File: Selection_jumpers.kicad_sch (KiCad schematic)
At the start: 7 parts, among them J10 U2RS485_TX, J17 U2RS485_DE_~{RE}, J17 U2RS485_RX, J6 R4_TX, J7 R4_RX

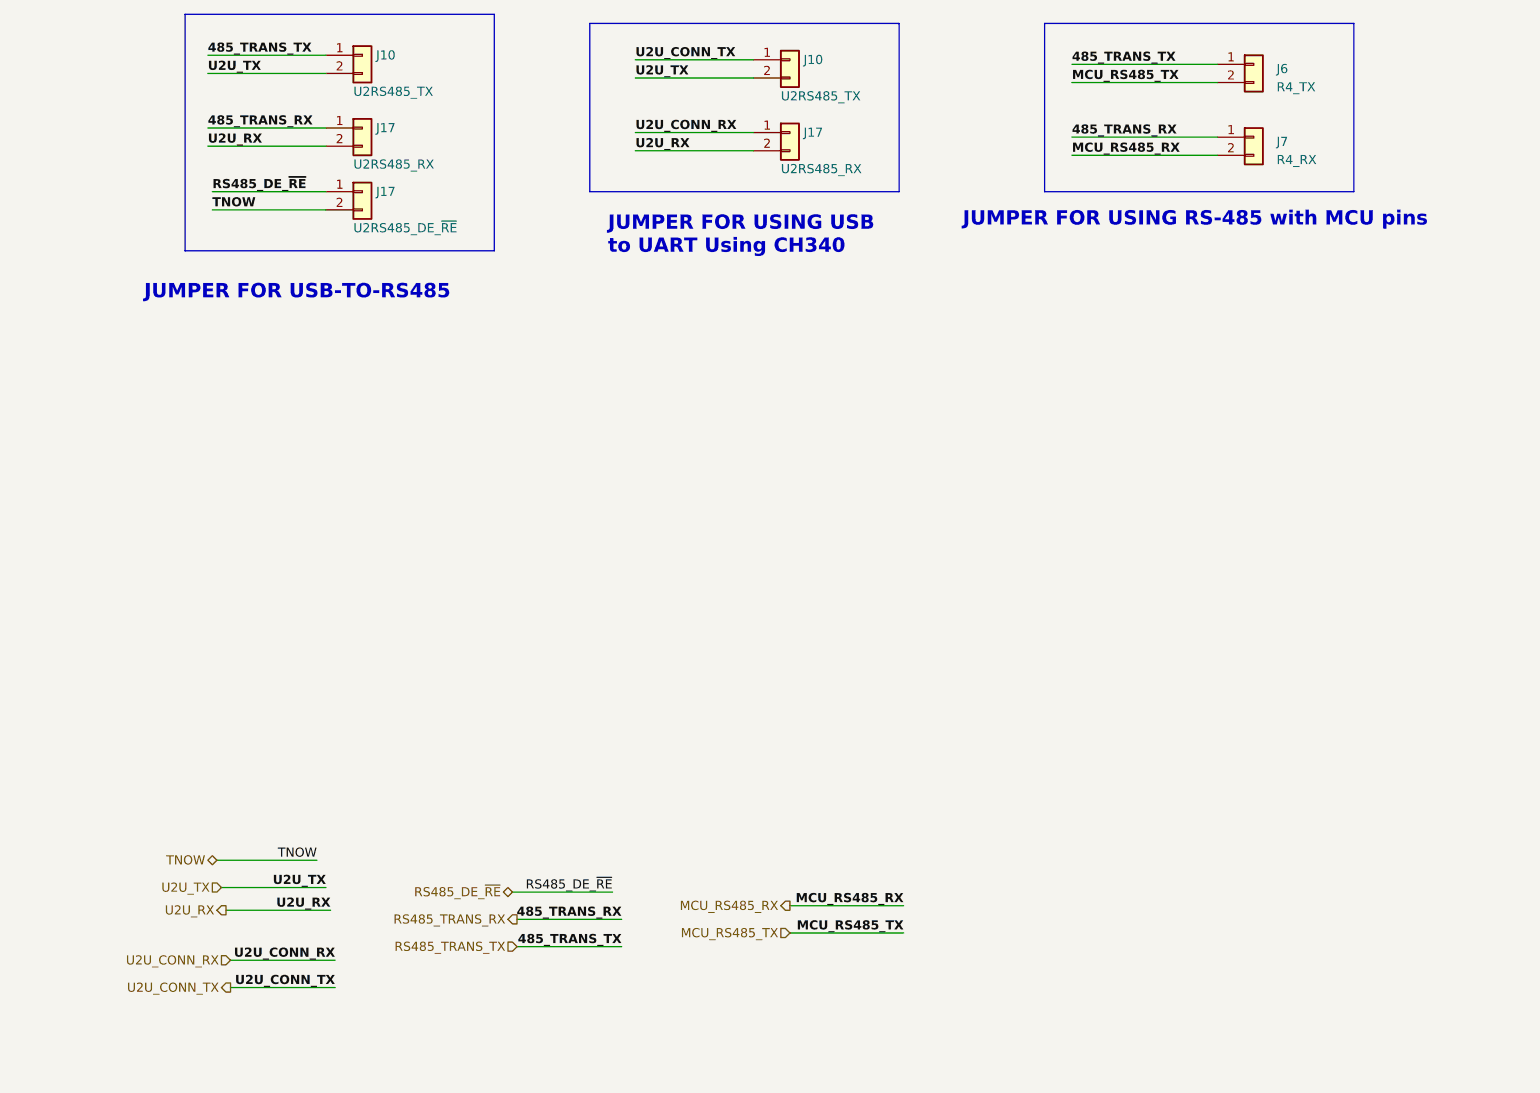
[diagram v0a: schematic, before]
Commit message: Merge changes upstream
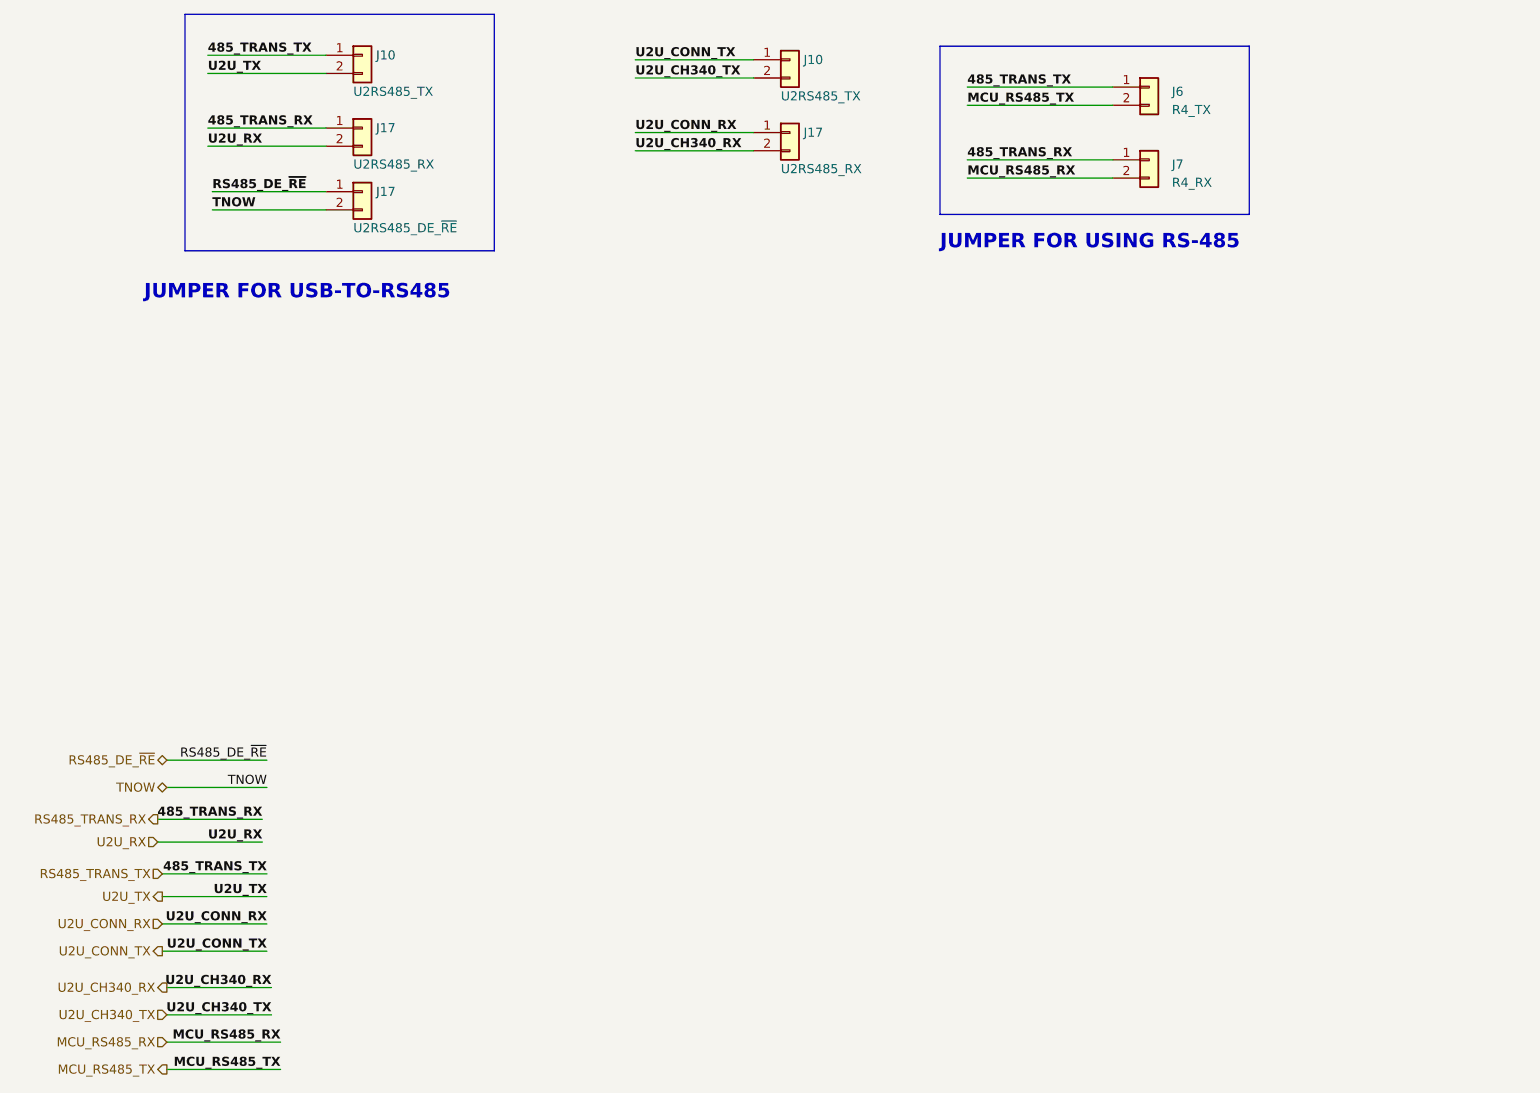
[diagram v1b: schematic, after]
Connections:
- net U2U_RX: no longer J17.2 (Pin_2)
- net U2U_TX: no longer J10.2 (Pin_2)
- new net U2U_CH340_RX: J17.2 (Pin_2)
- new net U2U_CH340_TX: J10.2 (Pin_2)
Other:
- note added: "JUMPER FOR USING RS-485"
- note removed: "JUMPER FOR USING RS-485 with MCU pins"
- note removed: "JUMPER FOR USING USB to UART Using CH340"
- moved on the sheet: J6, J7
